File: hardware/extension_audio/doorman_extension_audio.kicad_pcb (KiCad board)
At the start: 4 copper layers, 31.4 x 29.6 mm, 64 parts, among them J1 Output, J2 GPIO, J3 Input, J4 Extension Board Connector, U2 ES8311

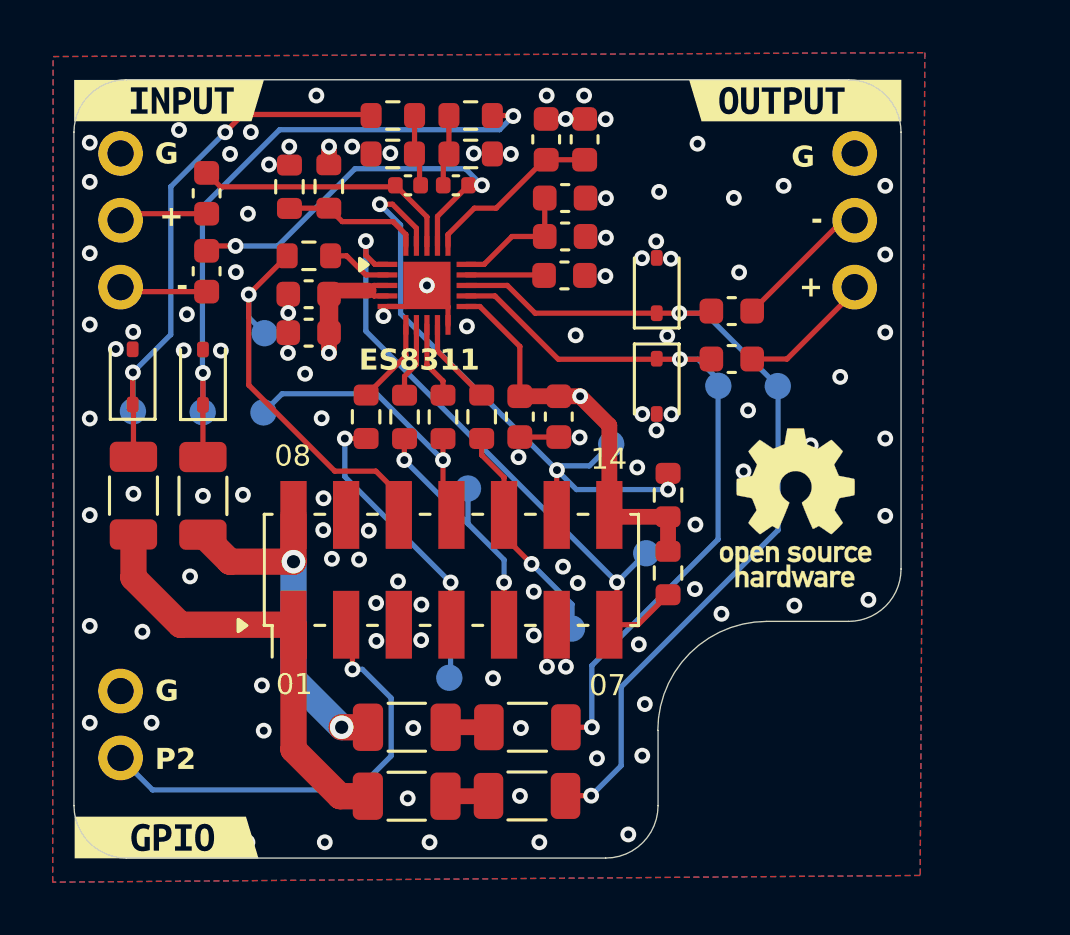
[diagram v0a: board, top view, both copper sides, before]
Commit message: WIP
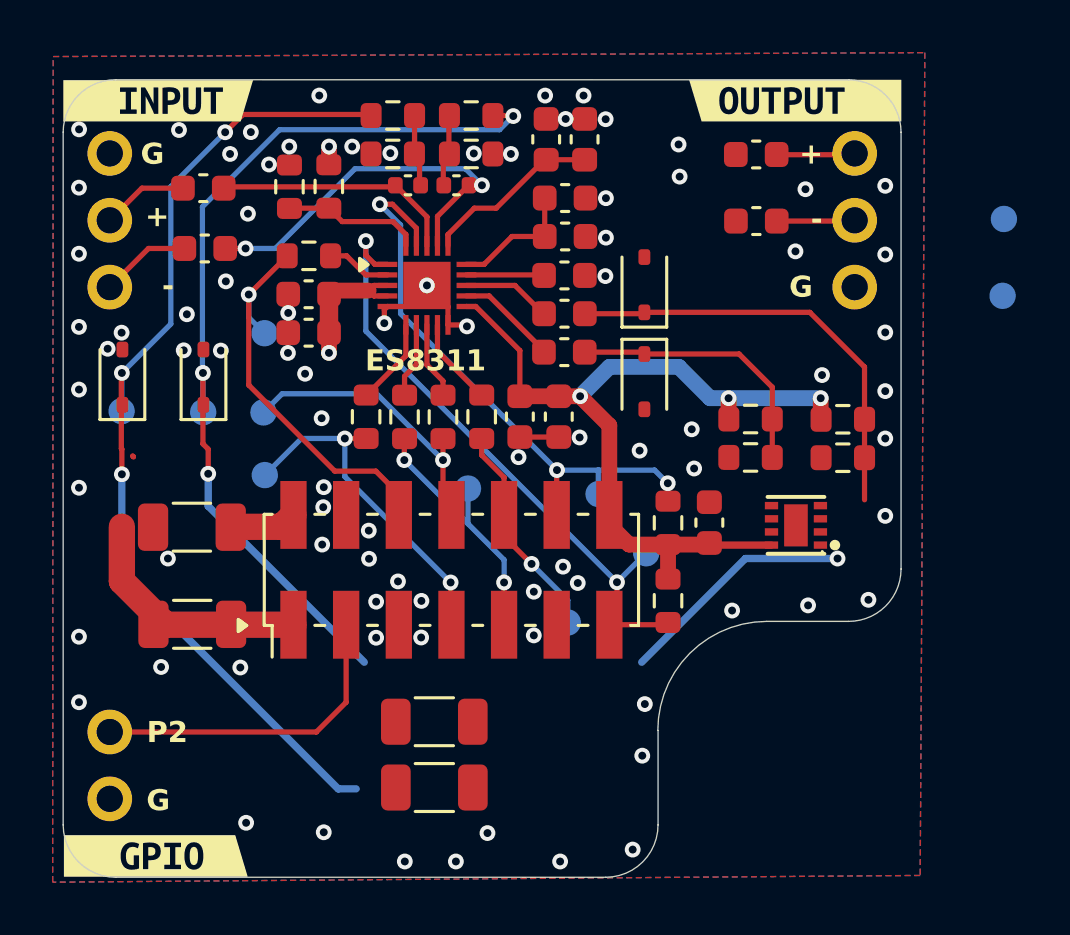
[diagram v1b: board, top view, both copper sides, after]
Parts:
- removed REF**: OSHW-Logo_5.7x6mm_SilkScreen, Symbol:OSHW-Logo_5.7x6mm_SilkScreen
- removed kibuzzard-69BBD06F: G***, kibuzzard-69BBD06F
- added C22: 100nF, Capacitor_SMD:C_0603_1608Metric, F.Cu at (107.5, 64.6)
- added R4: 10K, Resistor_SMD:R_0603_1608Metric, F.Cu at (109.0, 62.2)
- added R7: 10K, Resistor_SMD:R_0603_1608Metric, F.Cu at (109.0, 60.7)
- added R8: 10K, Resistor_SMD:R_0603_1608Metric, F.Cu at (112.5, 60.7)
- added R9: 10K, Resistor_SMD:R_0603_1608Metric, F.Cu at (112.5, 62.2)
- added U3: TLV9002IDSGR, Doorman:WSON-8_L2.0-W2.0-P0.65-BL-EP, F.Cu at (110.8, 64.7)
- added kibuzzard-69DCDFB0: G***, kibuzzard-69DCDFB0, B.Cu at (86.5, 48.6)
- C12, C4: value 10uF -> 2.2uF
- C14, C8: footprint Capacitor_SMD:C_1206_3216Metric -> Capacitor_SMD:C_0603_1608Metric
- J2: moved to F.Cu
- R10, R6: value 200 -> 150R
- R15, R16, R17, R18, R19: value 33 -> 33R
- moved C8 19.3 mm to (102.0, 56.7)
- moved C14 15.5 mm to (102.0, 58.2)
- moved TP4 11.3 mm to (118.6, 56.0)
- moved TP3 10.7 mm to (118.7, 53.1)
- moved TP8 10.4 mm to (90.6, 62.8)
- moved C5 7.83 mm to (109.3, 50.6)
- moved C12 5.38 mm to (87.8, 68.5), turned to 180 degrees
- moved J1 5.08 mm to (113.0, 50.6), turned to 0 degrees
- moved C3 3.55 mm to (109.3, 53.2)
- moved R6 3.54 mm to (97.0, 72.2)
- moved R10 3.53 mm to (97.0, 74.7), turned to 0 degrees
- moved TP6 1.96 mm to (103.3, 63.5)
- moved C4 1.26 mm to (87.8, 64.8), turned to 180 degrees
- moved J2 1.07 mm to (84.7, 72.6)
- moved R14 1.06 mm to (105.9, 67.6)
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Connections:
- C14 pad 1: BUS_WIRE2 -> AUDIO_OUT_P
- C14 pad 2: Net-(C14-Pad2) -> Net-(D4-K)
- C8 pad 1: BUS_WIRE1 -> AUDIO_OUT_N
- C8 pad 2: Net-(C8-Pad2) -> Net-(D2-K)
- D2 pad 1: AUDIO_OUT_N -> Net-(D2-K)
- D4 pad 1: AUDIO_OUT_P -> Net-(D4-K)
- R10 pad 1: AUDIO_OUT_N -> Net-(D1-K)
- R10 pad 2: Net-(C8-Pad2) -> Net-(U3A-IN1-)
- R6 pad 1: AUDIO_OUT_P -> Net-(U3B-IN2-)
- R6 pad 2: Net-(C14-Pad2) -> Net-(D3-K)
- TP3 pad 1: AUDIO_OUT_N -> Net-(D2-K)
- TP4 pad 1: AUDIO_OUT_P -> Net-(D4-K)
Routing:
- net AUDIO_OUT_N: track 34.1 -> 3.40 mm, vias 2 -> 0
- net AUDIO_OUT_P: track 28.3 -> 3.86 mm, vias 2 -> 0
- net Net-(D1-K): track 25.1 -> 44.5 mm, vias 2 -> 4
- net Net-(D3-K): track 21.1 -> 37.9 mm, vias 2 -> 3
- net Net-(D2-K): track 0.00 -> 16.6 mm
- net AVDD: track 39.7 -> 55.8 mm, vias 3 -> 5
- net BUS_WIRE1: track 13.7 -> 2.52 mm, vias 2 -> 0
- net Net-(D4-K): track 0.00 -> 10.4 mm
- net BUS_WIRE2: track 16.8 -> 9.28 mm
- net PIN2: track 18.0 -> 12.4 mm, vias 1 -> 0
- net Net-(J1-Pin_2): track 5.36 -> 2.97 mm
- net Net-(J1-Pin_1): track 5.40 -> 3.31 mm
- net Net-(C14-Pad2): track 1.64 -> 0.00 mm
- net Net-(C8-Pad2): track 1.64 -> 0.00 mm
- net I2C_DAT: track 24.7 -> 23.1 mm
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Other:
- board size 31.4 x 29.6 mm -> 31.8 x 30.3 mm
- board text removed: "01"
- board text removed: "07"
- board text removed: "08"
- board text removed: "14"
